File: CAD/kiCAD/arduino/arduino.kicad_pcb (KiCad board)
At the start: 2 copper layers, 33.9 x 65.8 mm, 8 parts

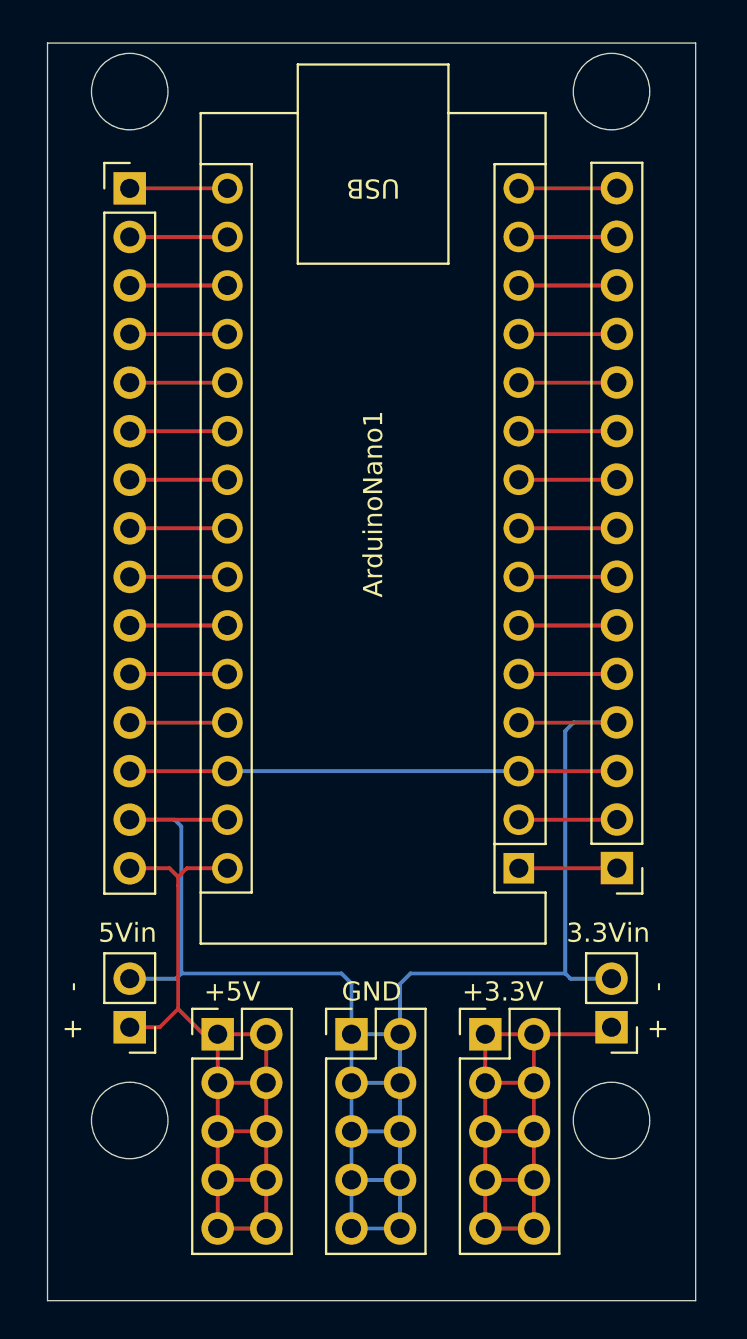
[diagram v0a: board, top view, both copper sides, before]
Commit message: updates
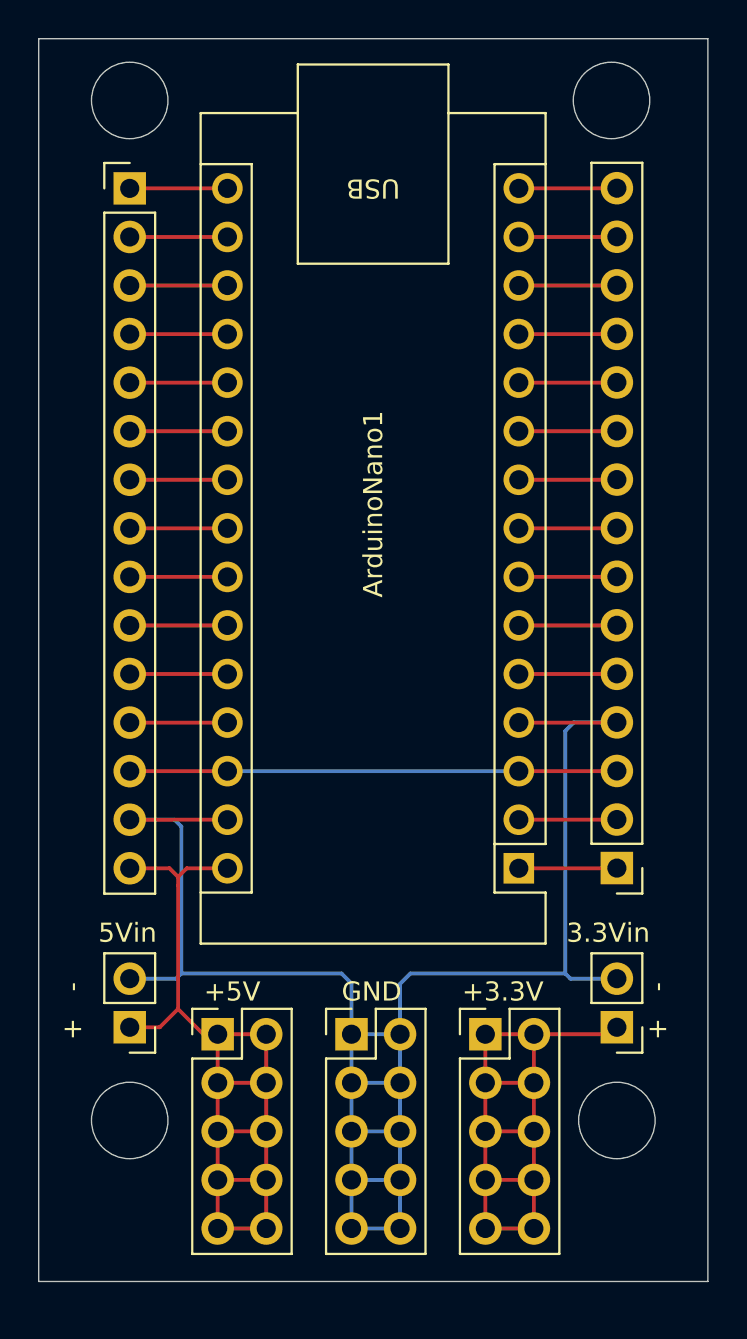
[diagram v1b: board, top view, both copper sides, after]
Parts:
- moved powerIN2 0.28 mm to (159.4, 117.6)
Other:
- board size 33.9 x 65.8 mm -> 35 x 65 mm
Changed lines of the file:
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@@
 		)
 		(property "Value" "Conn_02x05_Counter_Clockwise"
-			(at 1.27 12.49 360)
+			(at 1.27 12.49 0)
 			(layer "F.Fab")
 			(hide yes)
@@
 		)
 		(property "Value" "Conn_02x05_Counter_Clockwise"
-			(at 1.27 12.49 360)
+			(at 1.27 12.49 0)
 			(layer "F.Fab")
 			(hide yes)
@@
 		)
 		(property "Value" "Conn_01x02"
-			(at 0 7.5 360)
+			(at 0 7.5 0)
 			(layer "F.Fab")
 			(hide yes)
@@
 		(locked yes)
 		(layer "F.Cu")
-		(at 159.1 117.615 180)
+		(at 159.38 117.615 180)
 		(descr "Through hole straight pin header, 1x02, 2.54mm pitch, single row")
 		(tags "Through hole pin header THT 1x02 2.54mm single row")
 		(property "Reference" "powerIN2"
-			(at -1 -3.46 360)
+			(at -1 -3.46 0)
 			(layer "F.SilkS")
 			(hide yes)
@@
 		)
 		(property "Value" "Conn_01x02"
-			(at 0 4.87 360)
+			(at 0 4.87 0)
 			(layer "F.Fab")
 			(hide yes)
@@
 		)
 		(property "Value" "Conn_02x05_Counter_Clockwise"
-			(at 1.27 12.49 360)
+			(at 1.27 12.49 0)
 			(layer "F.Fab")
 			(hide yes)
@@
 	)
 	(footprint "Module:Arduino_Nano"
+		(locked yes)
 		(layer "F.Cu")
 		(at 154.25 109.3 180)
@@
 	)
 	(gr_circle
-		(center 159.1 122.49)
-		(end 161.1 122.49)
+		(center 159.38 122.49)
+		(end 161.38 122.49)
 		(stroke
 			(width 0.05)
@@
 	)
 	(gr_rect
-		(start 129.6 66.14)
-		(end 163.5 131.915)
+		(start 129.14 65.9116)
+		(end 164.14 130.9116)
 		(stroke
 			(width 0.05)
@@
 	)
 	(gr_circle
-		(center 159.1 68.6775)
-		(end 161.1 68.6775)
+		(center 159.1 69.14)
+		(end 161.1 69.14)
 		(stroke
 			(width 0.05)
@@
 	)
 	(gr_circle
-		(center 133.9 68.6775)
-		(end 135.9 68.6775)
+		(center 133.9 69.14)
+		(end 135.9 69.14)
 		(stroke
 			(width 0.05)
